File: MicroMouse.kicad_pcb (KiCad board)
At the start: 2 copper layers, 100 x 80 mm, 81 parts, among them CN1 mouseBattery, Q1 IRLML6402, Q2 IRLML6344, SW1 SPST, SW2 SPST, SW3 SPST, U1 STM32F405RGTx, U2 TB6612, U3 CN_MOTOR, U4 CN_MOTOR, U5 3p, U6 ICM-20602, U7 4p

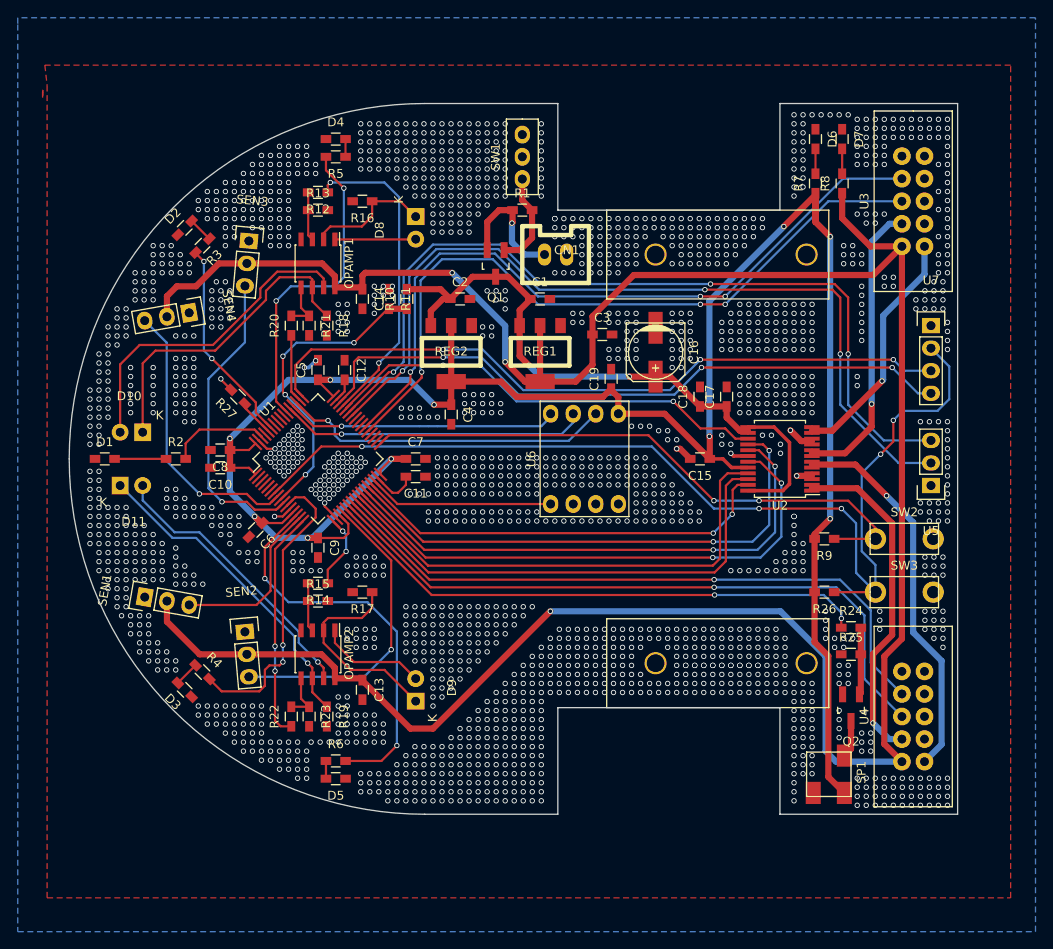
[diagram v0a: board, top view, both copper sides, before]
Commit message: とりあえず完成？
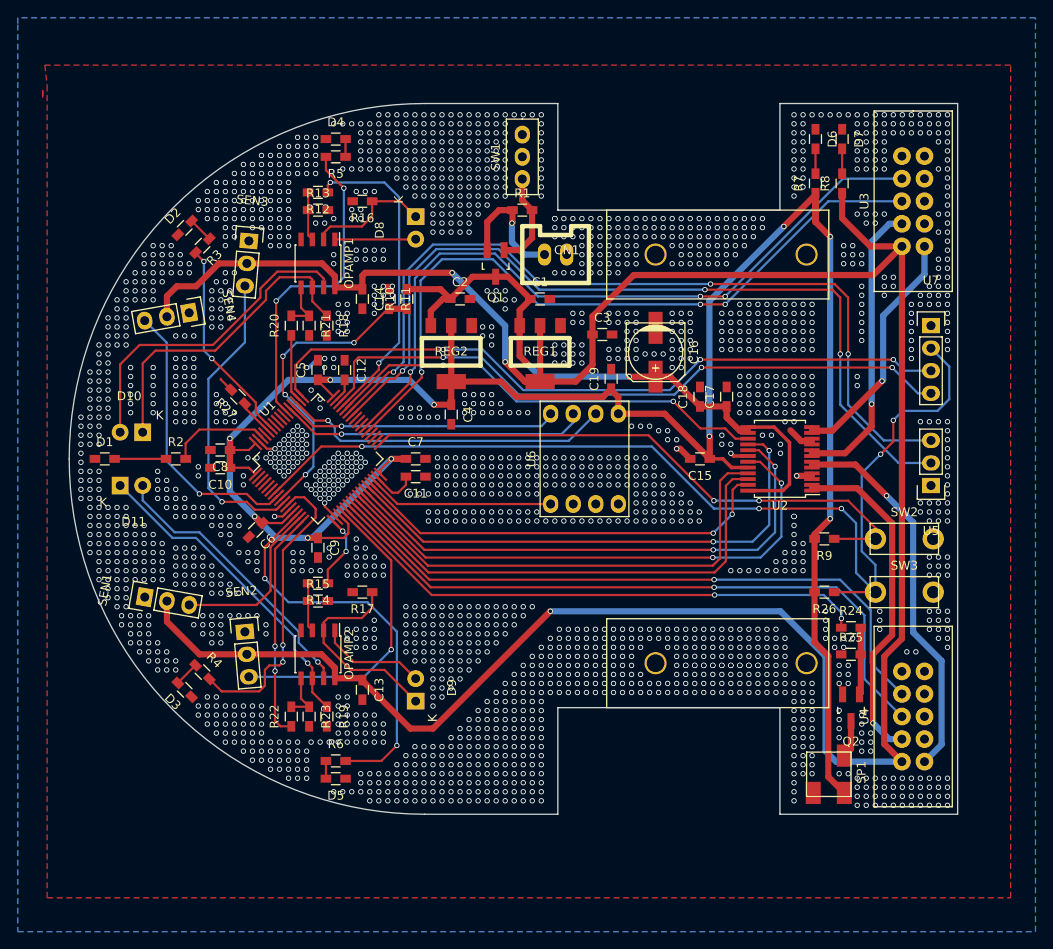
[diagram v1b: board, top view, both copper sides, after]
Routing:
- net GND: vias 2062 -> 2273
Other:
- rule trace_min: 0.203 -> 0.25

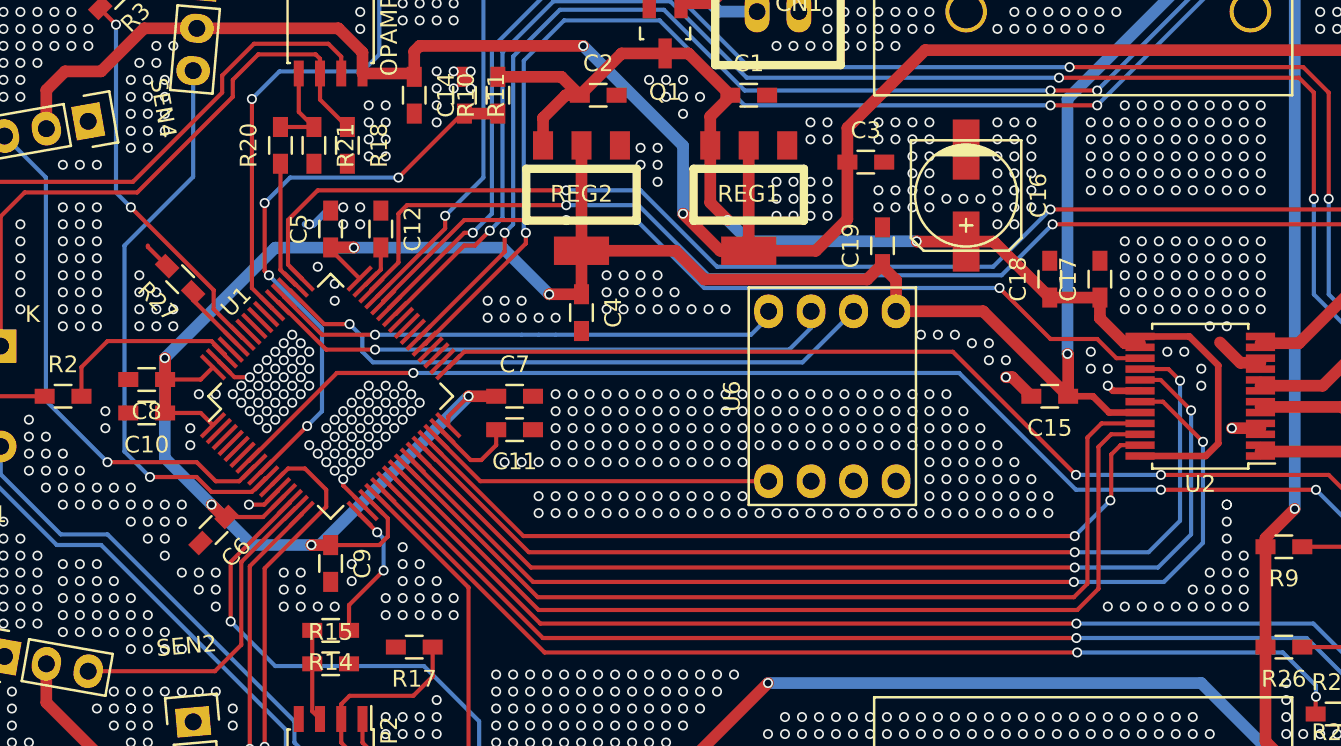
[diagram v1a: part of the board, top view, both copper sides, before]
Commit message: エンコーダ確認
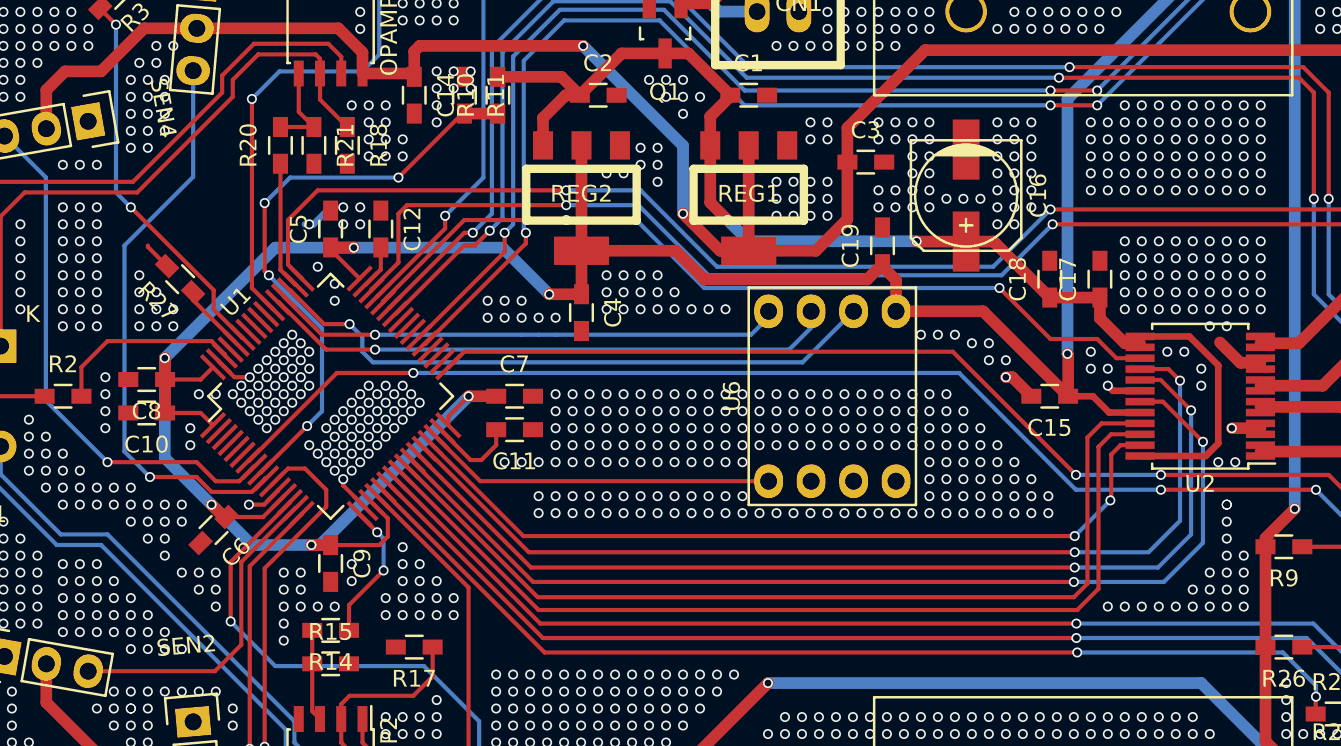
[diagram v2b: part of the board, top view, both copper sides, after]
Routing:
- net GND: vias 2273 -> 2284
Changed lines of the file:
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@@
     (thickness 1.6)
     (drawings 13)
-    (tracks 3002)
+    (tracks 3013)
     (zones 0)
     (modules 81)
@@
   (via (at 29.7688 17.018) (size 0.6) (drill 0.4) (layers F.Cu B.Cu) (net 2))
   (via (at 29.7688 18.034) (size 0.6) (drill 0.4) (layers F.Cu B.Cu) (net 2))
+  (via (at 81.0768 43.942) (size 0.6) (drill 0.4) (layers F.Cu B.Cu) (net 2))
+  (via (at 82.0928 43.942) (size 0.6) (drill 0.4) (layers F.Cu B.Cu) (net 2))
+  (via (at 14.5288 39.878) (size 0.6) (drill 0.4) (layers F.Cu B.Cu) (net 2))
+  (via (at 14.5288 38.862) (size 0.6) (drill 0.4) (layers F.Cu B.Cu) (net 2))
+  (via (at 44.5008 26.67) (size 0.6) (drill 0.4) (layers F.Cu B.Cu) (net 2))
+  (via (at 45.5168 26.67) (size 0.6) (drill 0.4) (layers F.Cu B.Cu) (net 2))
+  (via (at 29.2608 22.606) (size 0.6) (drill 0.4) (layers F.Cu B.Cu) (net 2))
+  (via (at 32.3088 24.638) (size 0.6) (drill 0.4) (layers F.Cu B.Cu) (net 2))
+  (via (at 32.3088 25.654) (size 0.6) (drill 0.4) (layers F.Cu B.Cu) (net 2))
+  (via (at 25.1968 53.594) (size 0.6) (drill 0.4) (layers F.Cu B.Cu) (net 2))
+  (via (at 25.1968 54.61) (size 0.6) (drill 0.4) (layers F.Cu B.Cu) (net 2))
   (segment (start 53 25) (end 53 31.3) (width 0.7) (layer F.Cu) (net 3) (status C00030))
   (segment (start 53 31.3) (end 57.0158 31.3) (width 0.7) (layer F.Cu) (net 3) (status 400010))
@@
       )
     )
+  )
+  (zone (net 0) (net_name "") (layer F.Cu) (hatch edge 0.508)
+    (connect_pads (clearance 0.508))
+    (min_thickness 0.254)
+    (keepout (tracks not_allowed) (vias not_allowed) (copperpour not_allowed))
+    (fill (arc_segments 32) (thermal_gap 0.508) (thermal_bridge_width 0.508))
+    (polygon
+      (pts
+        (xy 46.1391 17.4625) (xy 46.1391 18.796) (xy 47.0662 17.8689)
+      )
+    )
+  )
+  (zone (net 0) (net_name "") (layer F.Cu) (hatch edge 0.508)
+    (connect_pads (clearance 0.508))
+    (min_thickness 0.254)
+    (keepout (tracks not_allowed) (vias not_allowed) (copperpour not_allowed))
+    (fill (arc_segments 32) (thermal_gap 0.508) (thermal_bridge_width 0.508))
+    (polygon
+      (pts
+        (xy 45.2628 18.6563) (xy 43.7007 18.6563) (xy 43.7007 19.8374)
+      )
+    )
+  )
+  (zone (net 0) (net_name "") (layer F.Cu) (hatch edge 0.508)
+    (connect_pads (clearance 0.508))
+    (min_thickness 0.254)
+    (keepout (tracks not_allowed) (vias not_allowed) (copperpour not_allowed))
+    (fill (arc_segments 32) (thermal_gap 0.508) (thermal_bridge_width 0.508))
+    (polygon
+      (pts
+        (xy 62.9666 35.7505) (xy 62.9666 36.8173) (xy 61.4807 36.8173)
+      )
+    )
+  )
+  (zone (net 0) (net_name "") (layer F.Cu) (hatch edge 0.508)
+    (connect_pads (clearance 0.508))
+    (min_thickness 0.254)
+    (keepout (tracks not_allowed) (vias not_allowed) (copperpour not_allowed))
+    (fill (arc_segments 32) (thermal_gap 0.508) (thermal_bridge_width 0.508))
+    (polygon
+      (pts
+        (xy 70.1929 19.9644) (xy 70.1929 21.59) (xy 71.8185 19.9644)
+      )
+    )

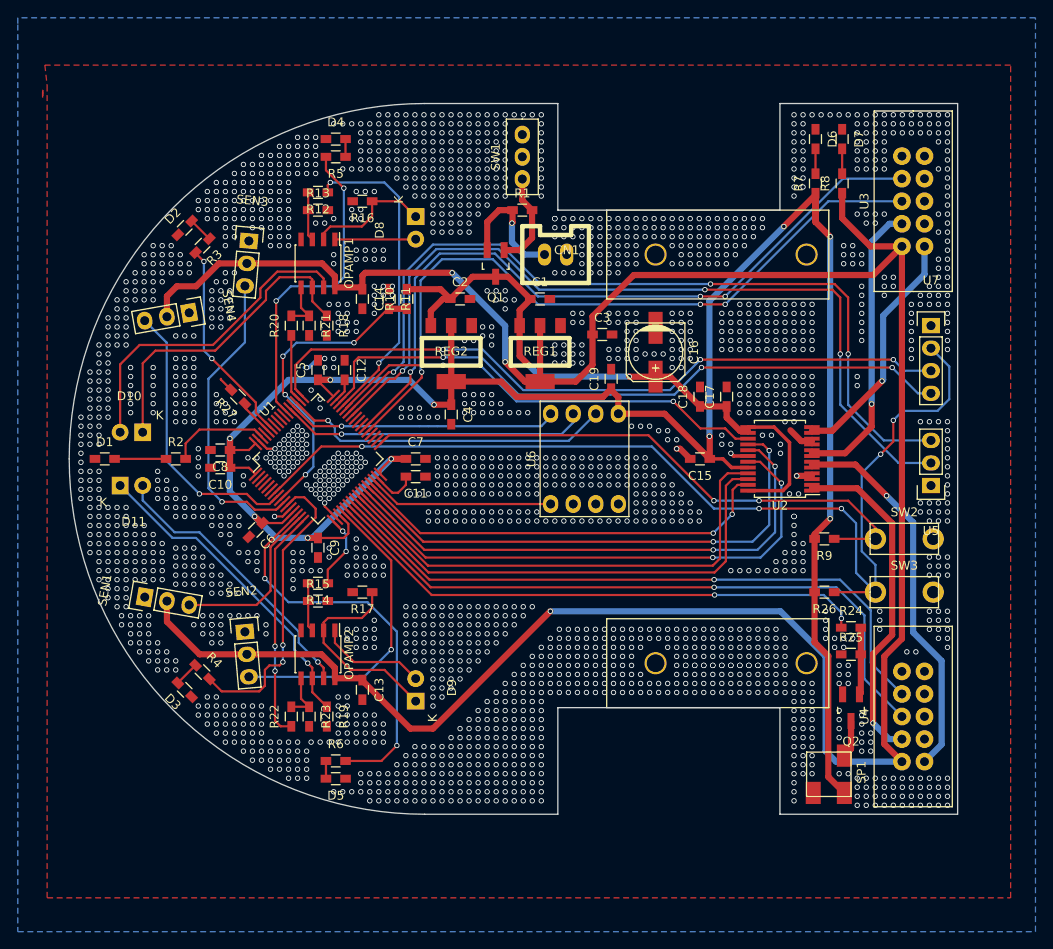
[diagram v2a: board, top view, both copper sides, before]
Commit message: 最終確認
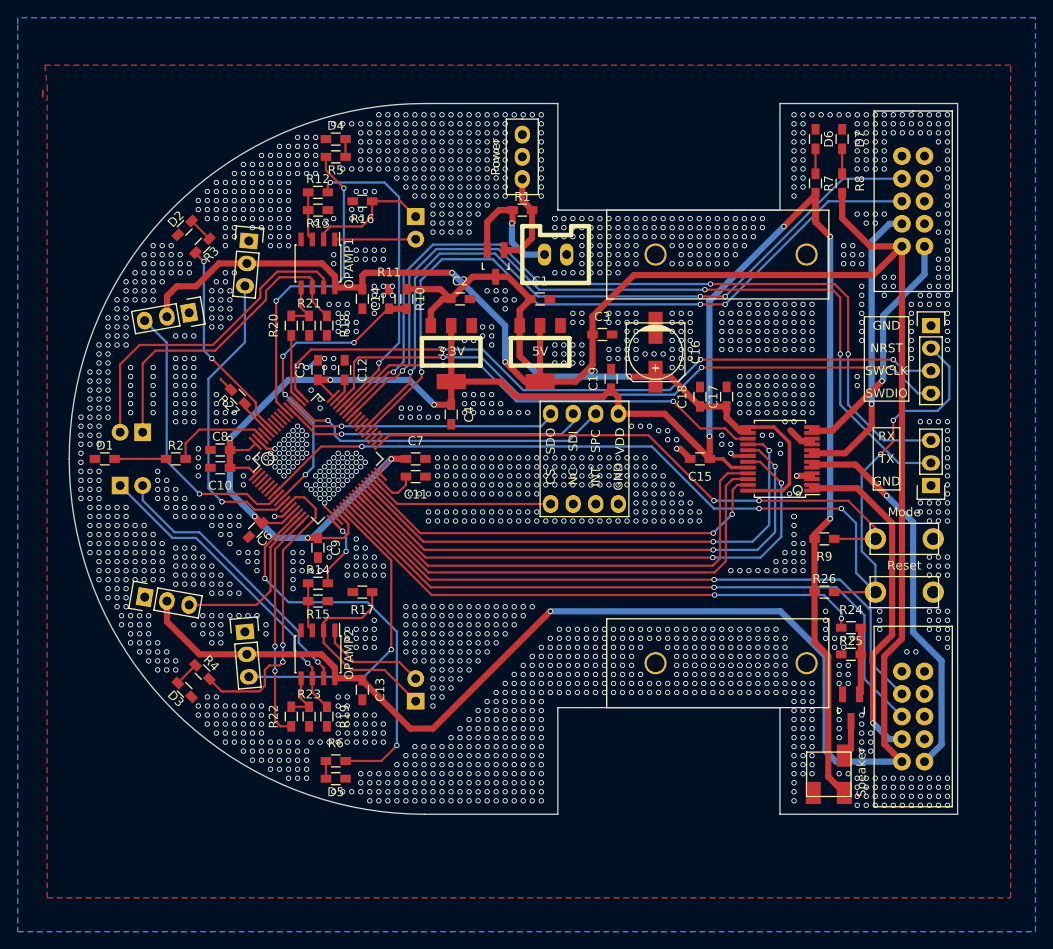
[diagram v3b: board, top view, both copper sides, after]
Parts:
- added REF**: serial, myfootprint:serial, F.Cu at (92.0, 40.0)
- added REF**: serial, myfootprint:serial, F.Cu at (92.0, 25.0)
- renumbered REG2 to 3.3V, REG1 to 5V, SW2 to Mode, SW1 to Power, SW3 to Reset, SP1 to Speaker
